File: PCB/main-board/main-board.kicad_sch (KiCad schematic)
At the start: 33 parts, among them J1 Conn_01x02_Pin, Q1 PN2222A, SW1 RotaryEncoder_Switch_MP, U1 LM358, U2 IRLIZ44N, U3 L7805

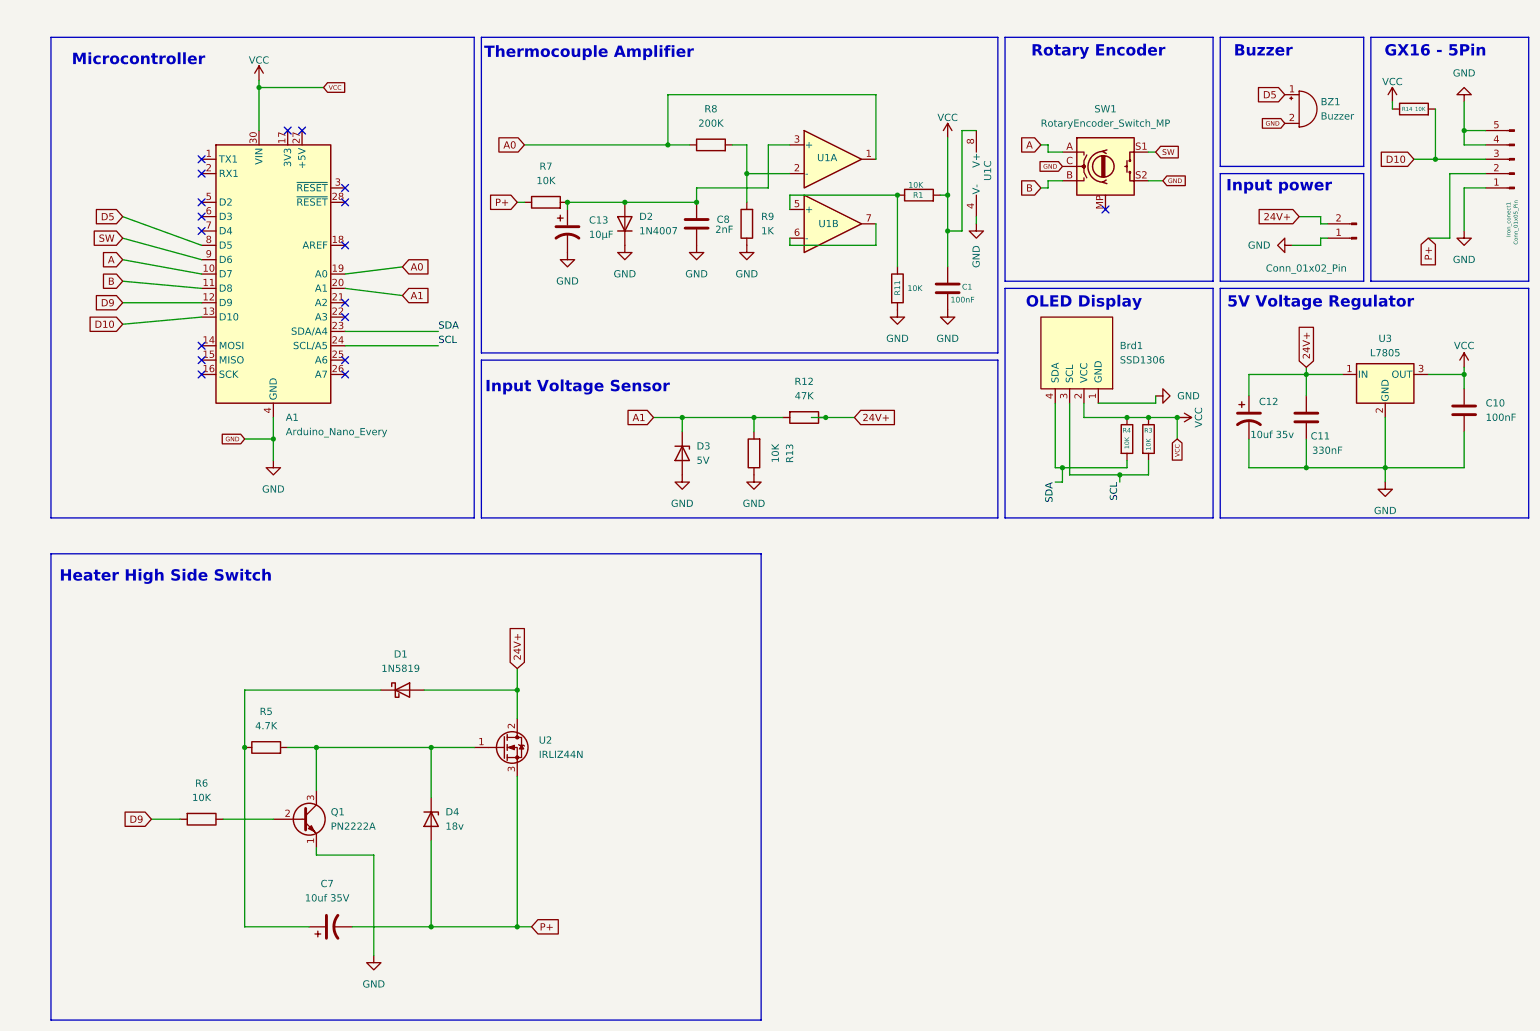
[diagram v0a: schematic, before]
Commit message: updated PCB files
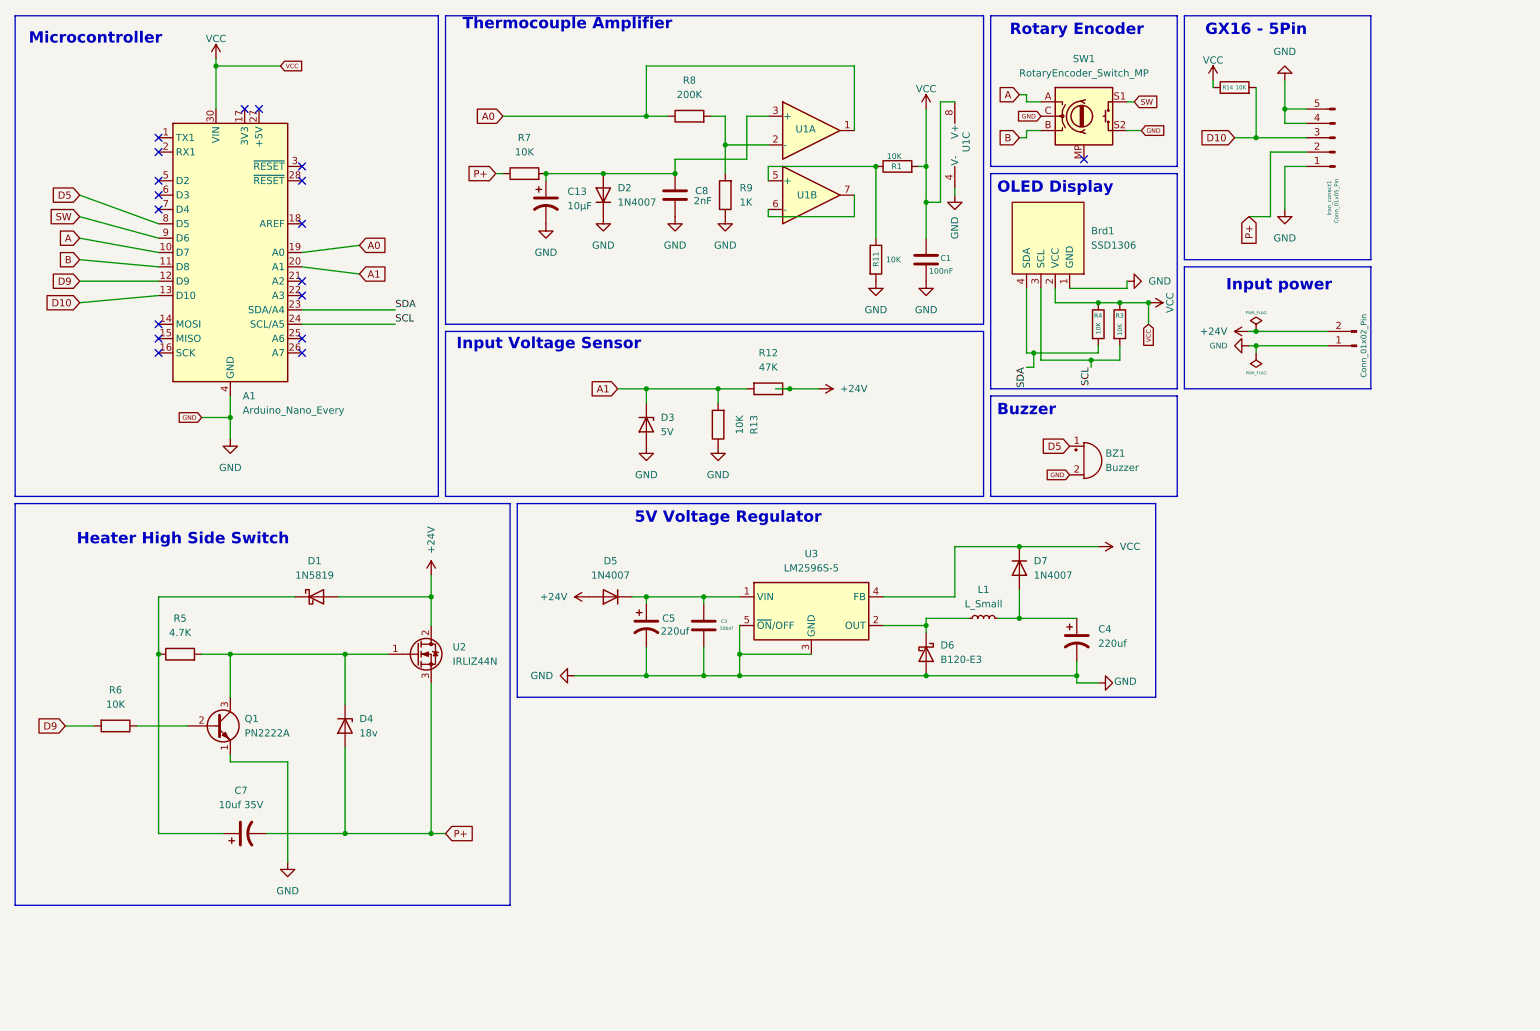
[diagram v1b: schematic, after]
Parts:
- removed C10: 100nF, Capacitor_SMD:C_0402_1005Metric, symbol Device:C
- removed C11: 330nF, Capacitor_SMD:C_0603_1608Metric, symbol Device:C
- removed C12: 10uf 35v, Capacitor_SMD:CP_Elec_5x4.4, symbol Device:C_Polarized_US
- removed U3: L7805, Package_TO_SOT_THT:TO-220F-3_Vertical, symbol Regulator_Linear:L7805
- added C3: 100nf, Capacitor_SMD:C_0402_1005Metric, symbol Device:C
- added C4, C5: 220uf, Capacitor_SMD:CP_Elec_8x10, symbol Device:C_Polarized_US
- added D5, D7: 1N4007, Diode_THT:D_DO-41_SOD81_P10.16mm_Horizontal, symbol Diode:1N4007
- added D6: B120-E3, Diode_SMD:D_SMA, symbol Diode:B120-E3
- added L1: L_Small, symbol Device:L_Small
- added U3: LM2596S-5, Package_TO_SOT_SMD:TO-263-5_TabPin3, symbol Regulator_Switching:LM2596S-5
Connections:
- net GND: now also C3.2, C4.2, C5.2, D6.2 (A), U3.3 (GND), U3.5 (~{ON}/OFF)
- net VCC: now also D7.1 (K), U3.4 (FB)
- net 24V+ renamed +24V
- net +24V: now also D5.2 (A)
- new net: C3.1, C5.1, D5.1 (K), U3.1 (VIN)
- new net: D6.1 (K), L1.1, U3.2 (OUT)
- new net: C4.1, D7.2 (A), L1.2
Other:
- moved on the sheet: A1, BZ1, Brd1, C1, C13, C7, C8, D1, D2, D3, D4, Iron_conect1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
